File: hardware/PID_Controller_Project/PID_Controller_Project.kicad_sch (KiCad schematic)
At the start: 38 parts, among them J1 Screw_Terminal_01x02, J2 Screw_Terminal_01x02, J3 Conn_01x04_Pin, M1 Fan, Q1 Q_NMOS_GDSD, Q2 Q_NMOS_GDSD, Q3 2N7000, SW1 RotaryEncoder_Switch, SW2 SW_Push, U1 STM32L476RGTx, U2 LCD-016N002L, U3 PCF8574AT, U4 BMP280

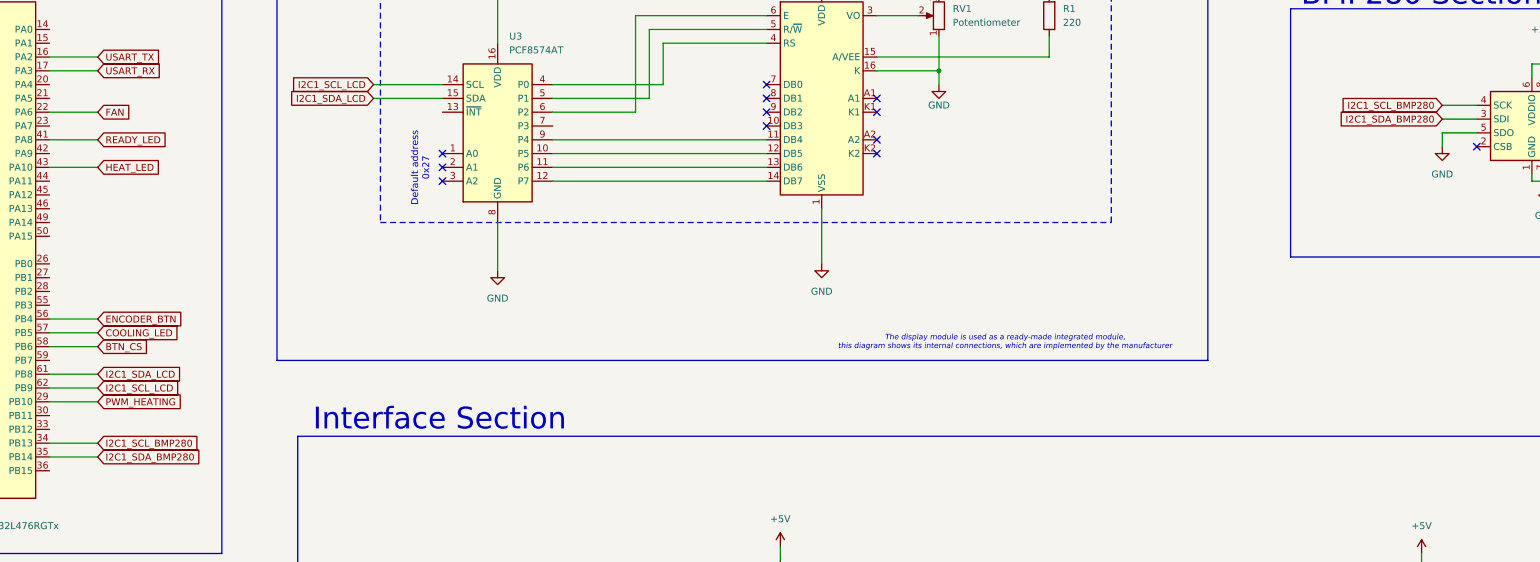
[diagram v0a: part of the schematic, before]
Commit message: correct schema
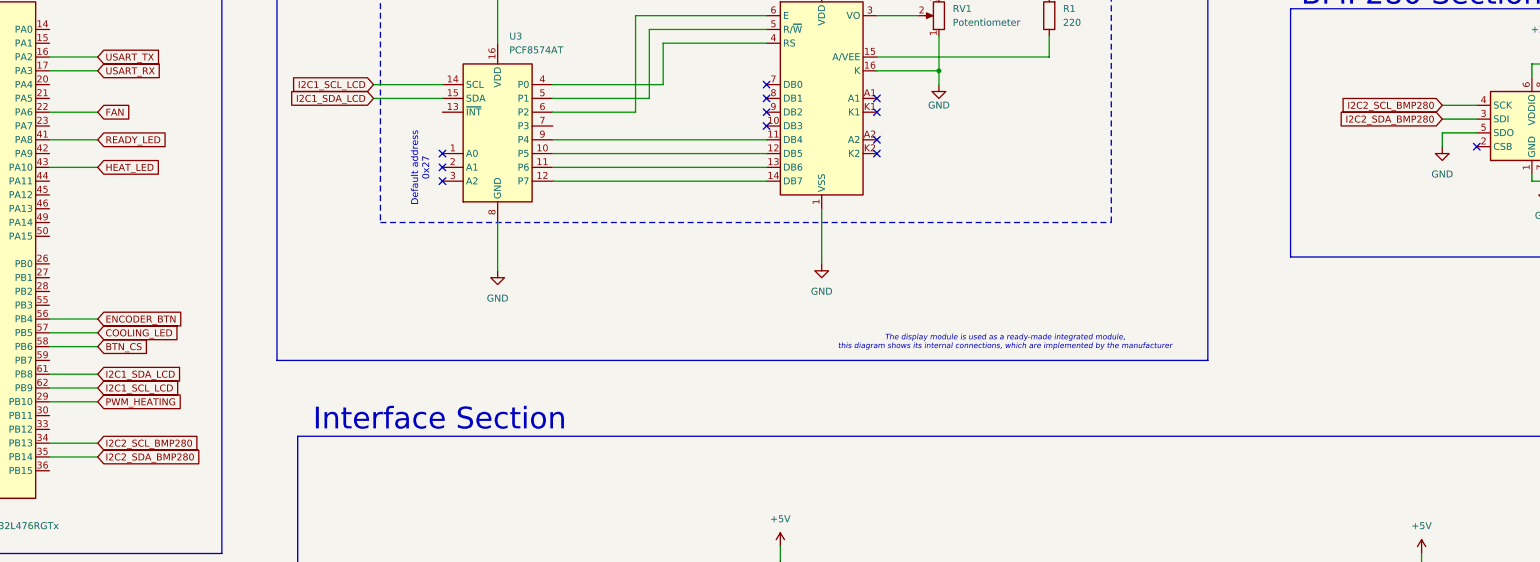
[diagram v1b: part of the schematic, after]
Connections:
- net I2C1_SCL_BMP280 renamed I2C2_SCL_BMP280
- net I2C1_SDA_BMP280 renamed I2C2_SDA_BMP280
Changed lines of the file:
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@@
 		)
 	)
-	(global_label "I2C1_SCL_BMP280"
+	(global_label "I2C2_SCL_BMP280"
 		(shape input)
 		(at 349.25 67.31 180)
@@
 		)
 	)
-	(global_label "I2C1_SDA_BMP280"
+	(global_label "I2C2_SDA_BMP280"
 		(shape input)
 		(at 101.6 132.08 0)
@@
 		)
 	)
-	(global_label "I2C1_SCL_BMP280"
+	(global_label "I2C2_SCL_BMP280"
 		(shape input)
 		(at 101.6 129.54 0)
@@
 		)
 	)
-	(global_label "I2C1_SDA_BMP280"
+	(global_label "I2C2_SDA_BMP280"
 		(shape input)
 		(at 349.25 69.85 180)

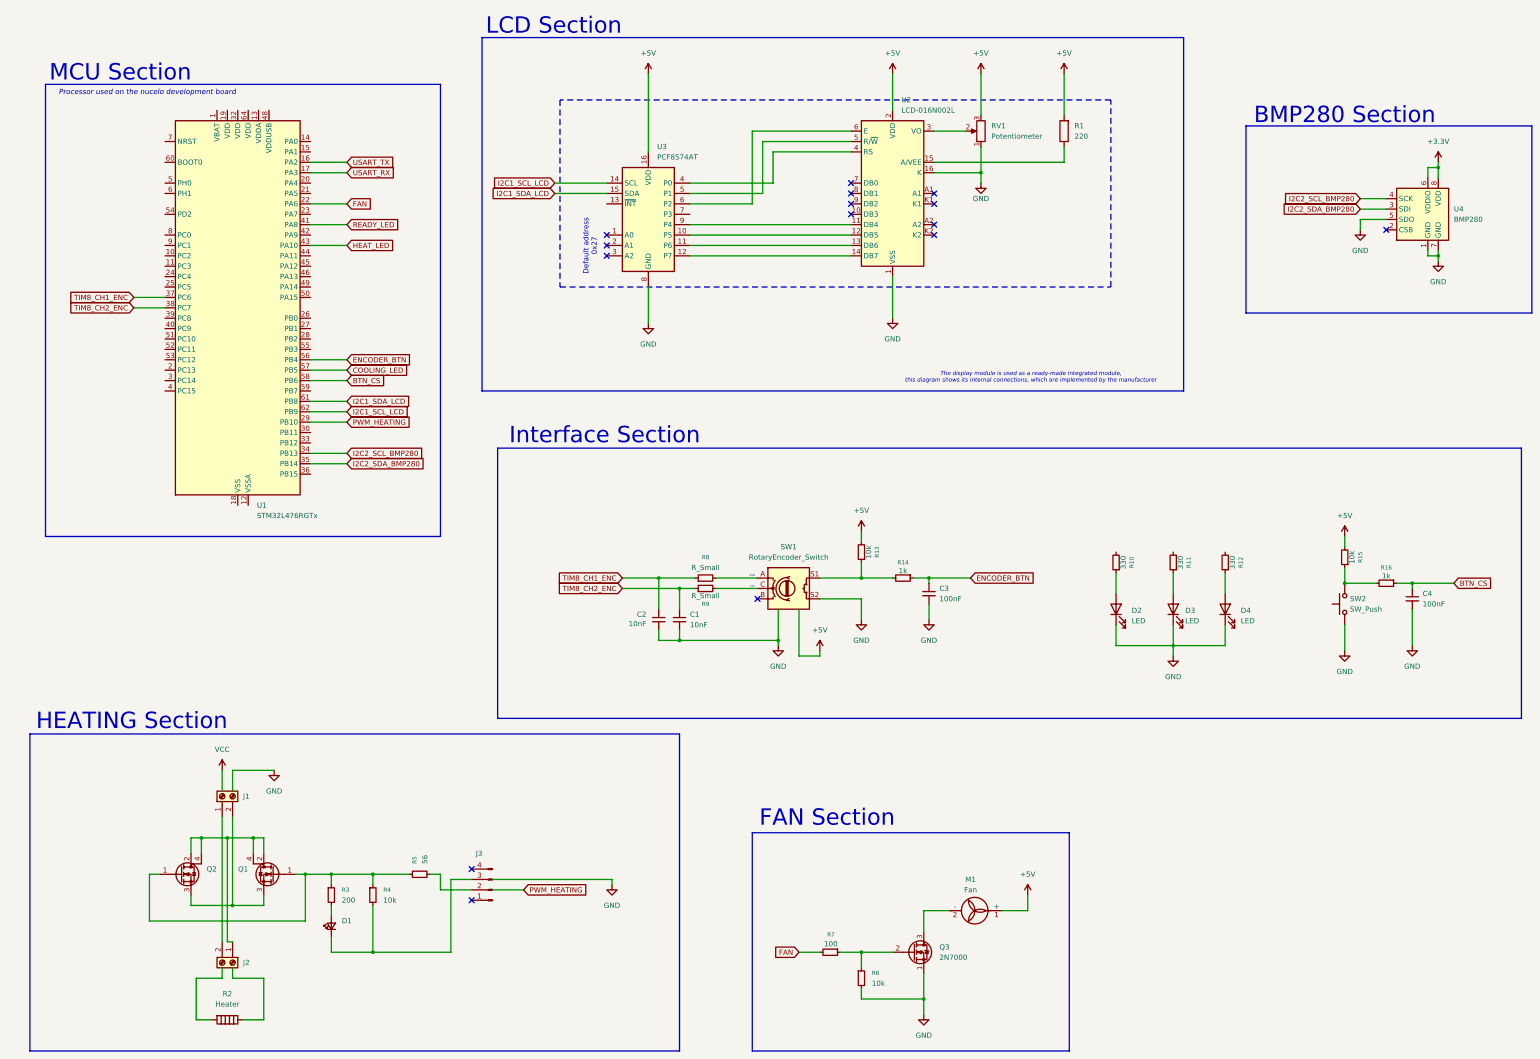
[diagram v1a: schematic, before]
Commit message: update schema
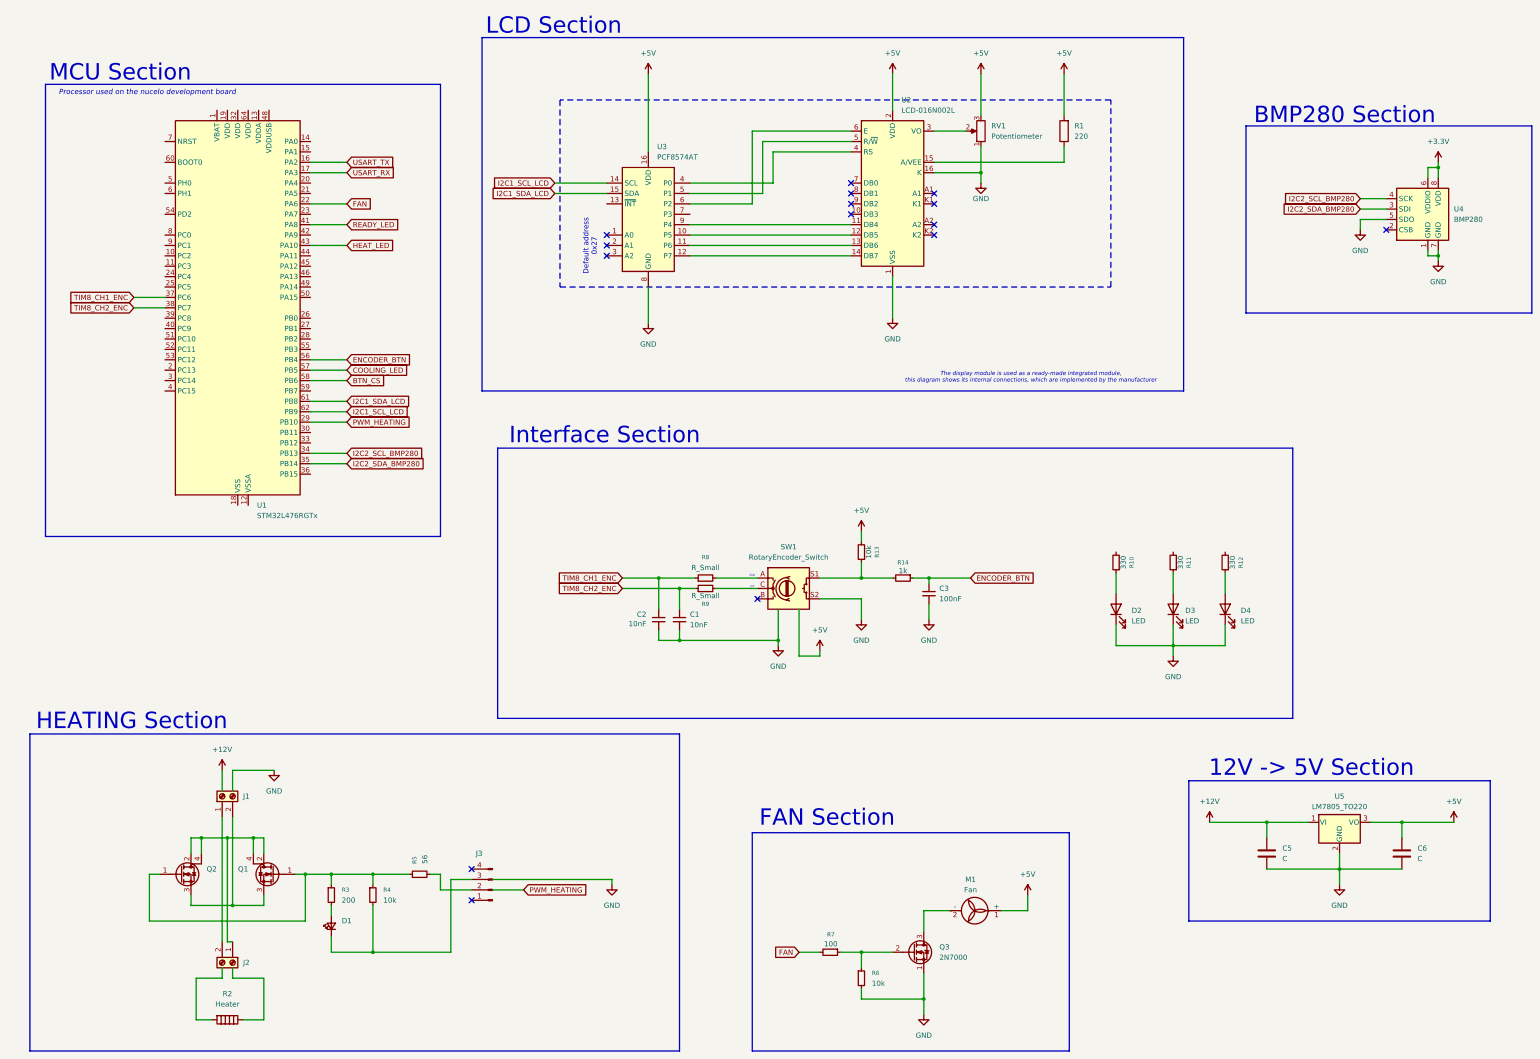
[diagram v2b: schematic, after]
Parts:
- removed C4: 100nF, symbol Device:C_Small
- removed R15: 10k, symbol Device:R_Small
- removed R16: 1k, symbol Device:R_Small
- removed SW2: SW_Push, symbol Switch:SW_Push
- added C5, C6: C, symbol Device:C
- added U5: LM7805_TO220, Package_TO_SOT_THT:TO-220-3_Vertical, symbol Regulator_Linear:LM7805_TO220
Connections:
- net +5V: now also C6.1, U5.3 (VO)
- net GND: now also C5.2, C6.2, U5.2 (GND)
- new net +12V: C5.1, U5.1 (VI)
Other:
- note added: "12V -> 5V Section"
